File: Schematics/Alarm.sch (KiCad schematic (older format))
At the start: 7 parts, among them U8 BluetoothModule, U9 Arduino

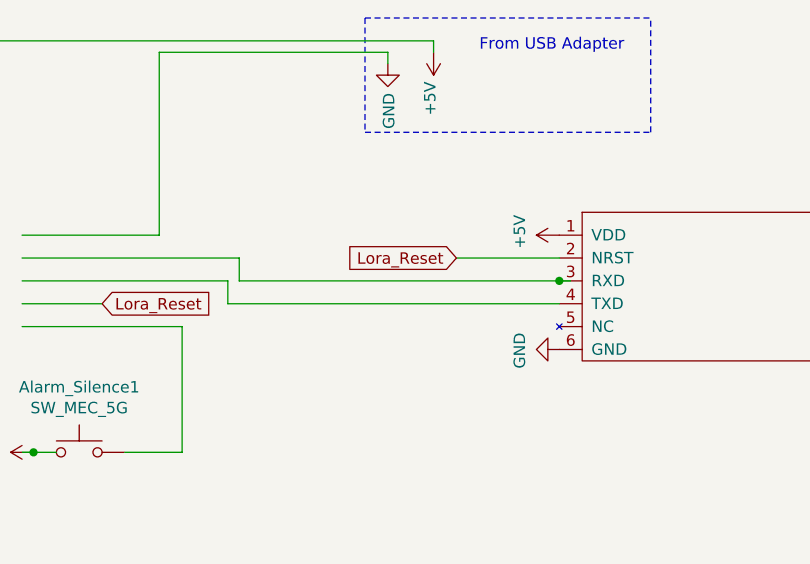
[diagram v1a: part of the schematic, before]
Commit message: Fixed a layer
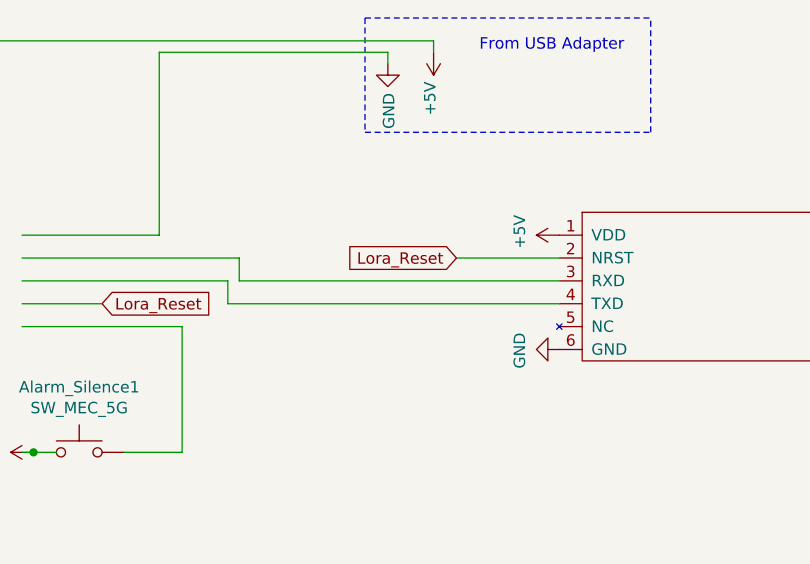
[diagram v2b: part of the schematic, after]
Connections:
- wire segments 37 -> 36
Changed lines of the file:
@@
 	4050 2800 4050 3400
 Wire Wire Line
-	7450 3400 7400 3400
-Wire Wire Line
 	6000 3400 6000 3300
-Connection ~ 7400 3400
-Wire Wire Line
-	7400 3400 6000 3400
 Wire Wire Line
 	5950 3400 5950 3500
@@
 Wire Wire Line
 	5050 3200 5650 3200
+Wire Wire Line
+	6000 3400 7400 3400
 $EndSCHEMATC

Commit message: Fixed repo
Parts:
- removed U9: Arduino, symbol CapstoneSchematic:Arduino
- added XA?: Arduino_Mega2560_Shield, symbol CapstoneSchematic:Arduino_Mega2560_Shield
- renumbered Alarm_Silence1 to Alarm_Silence, BZ1 to BZ?, D_RED2 to D_RED?, R4 to R?, U8 to U?, ULoRa2 to ULoRa?
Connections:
- wire segments 36 -> 56
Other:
- moved on the sheet: Alarm_Silence, BZ?, D_RED?, R?, U?, ULoRa?

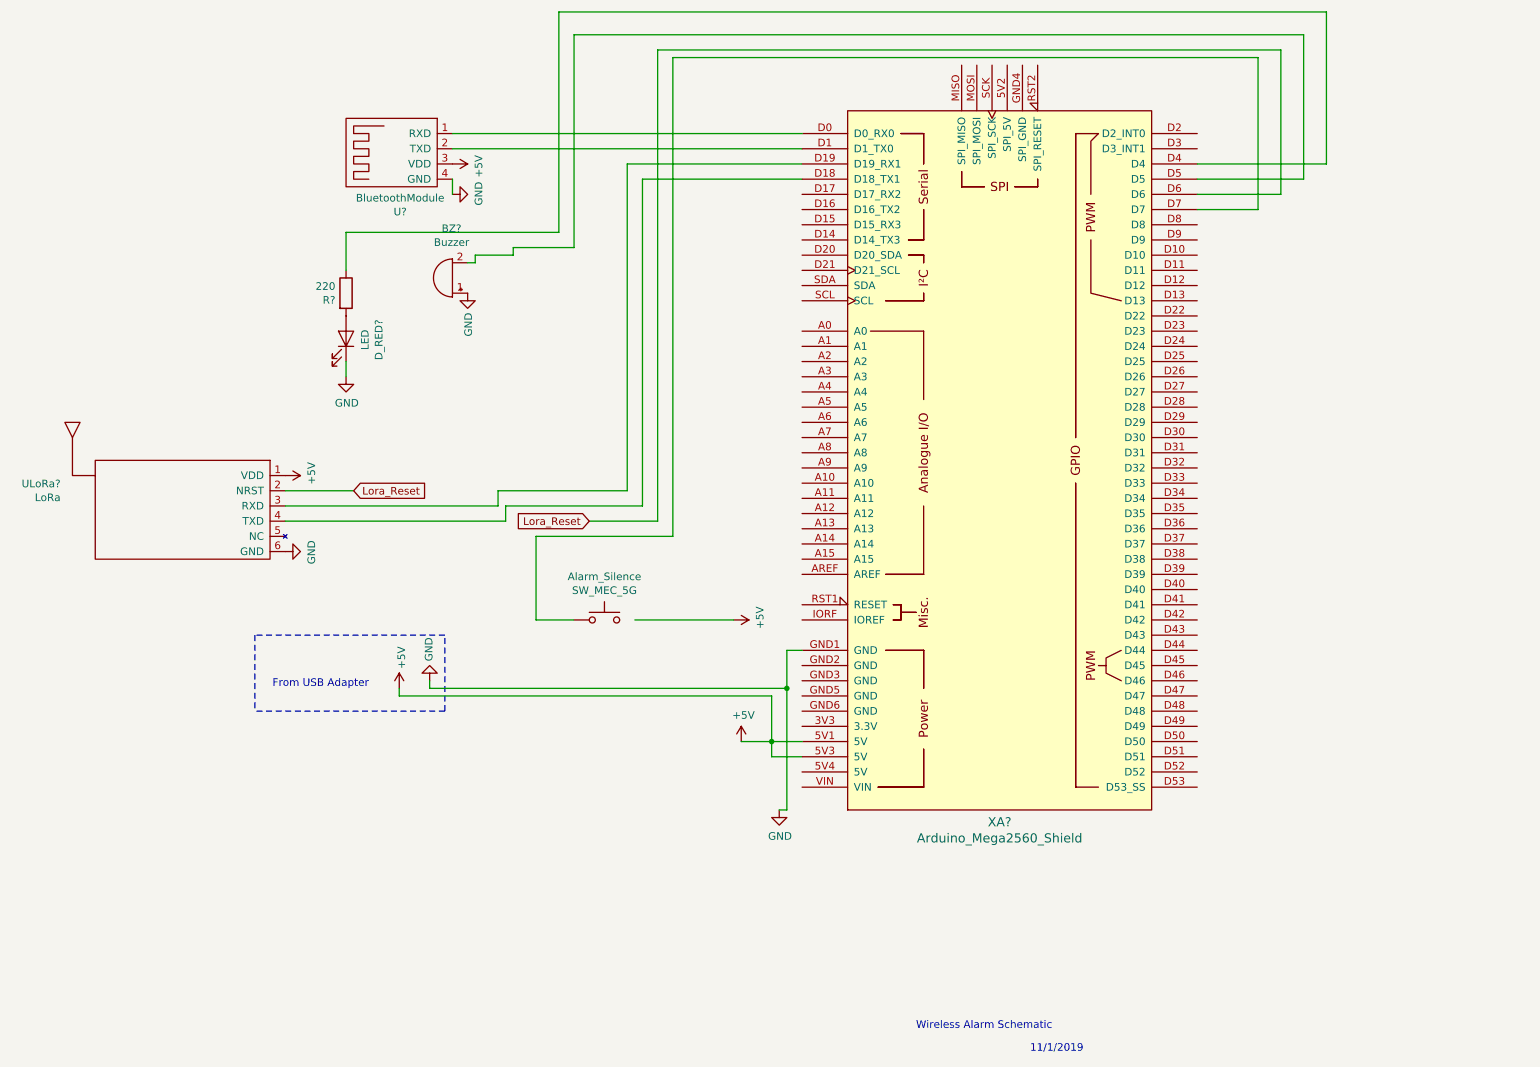
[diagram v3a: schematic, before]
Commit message: Made things look better on wireless alarm
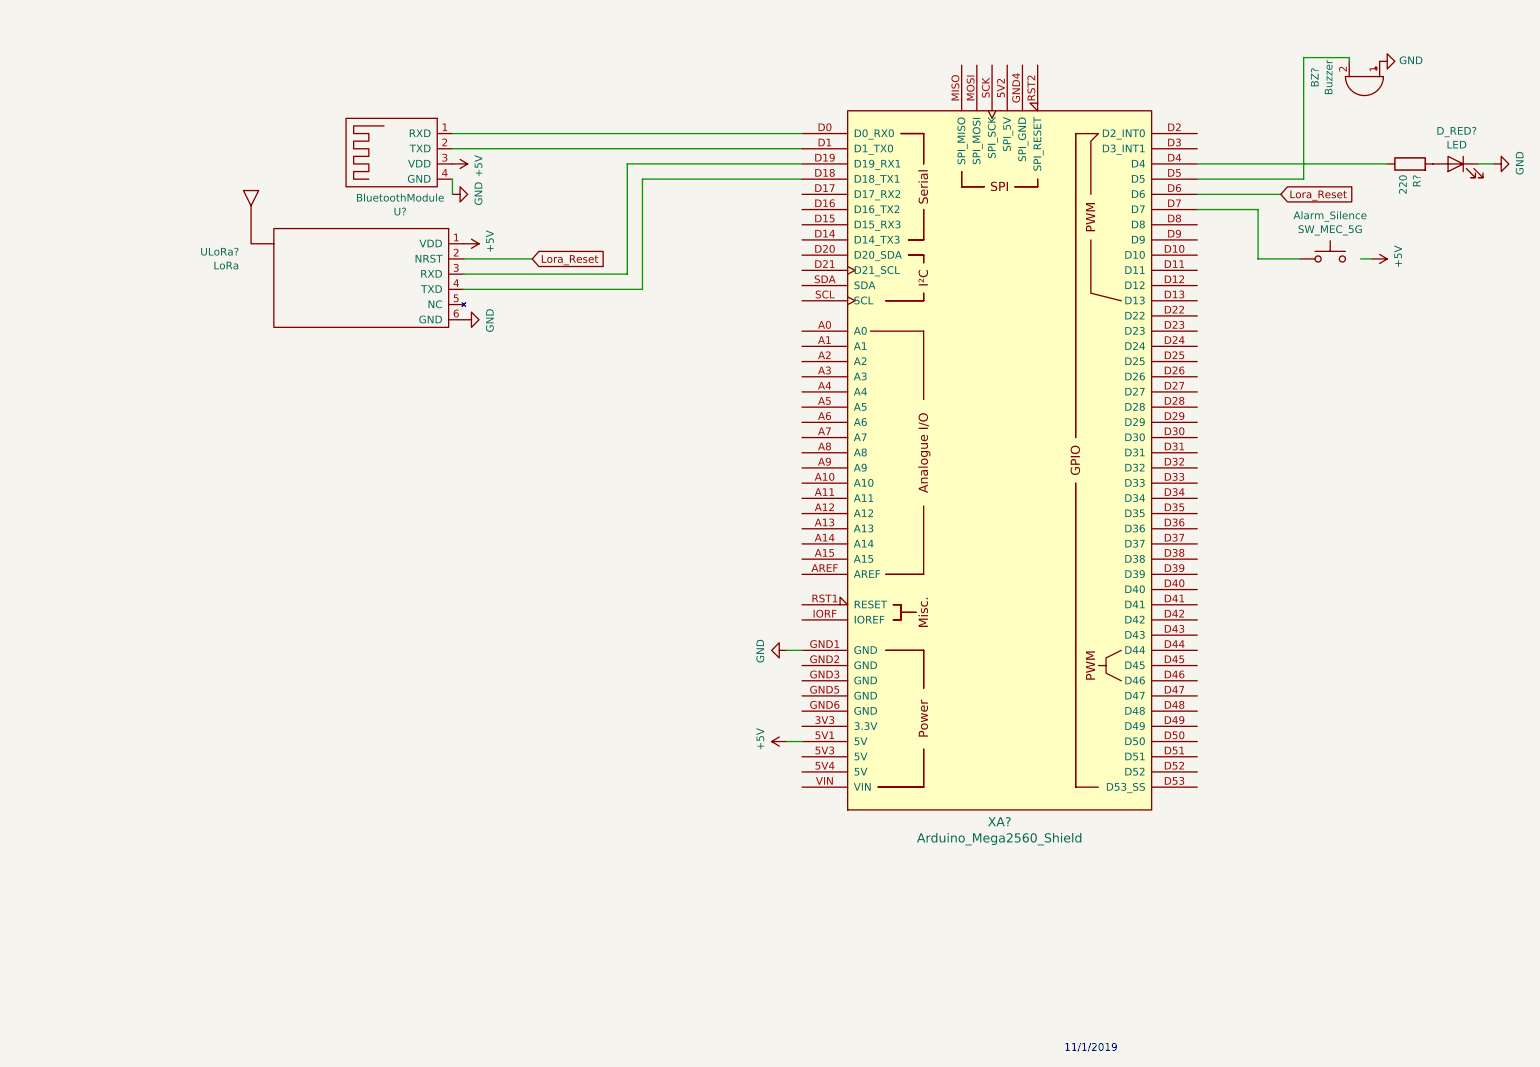
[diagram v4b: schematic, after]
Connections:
- net +5V: no longer XA?.5V3 (5V)
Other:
- note removed: "From USB Adapter"
- note removed: "Wireless Alarm Schematic"
- moved on the sheet: Alarm_Silence, BZ?, D_RED?, R?, ULoRa?
